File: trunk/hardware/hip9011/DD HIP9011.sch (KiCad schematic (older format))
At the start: 34 parts, among them P1 KNOCK 1, P2 KNOCK 2, P3 12V, P4 CONN_4X2, U1 7805-SOT89, X1 QUARTZ

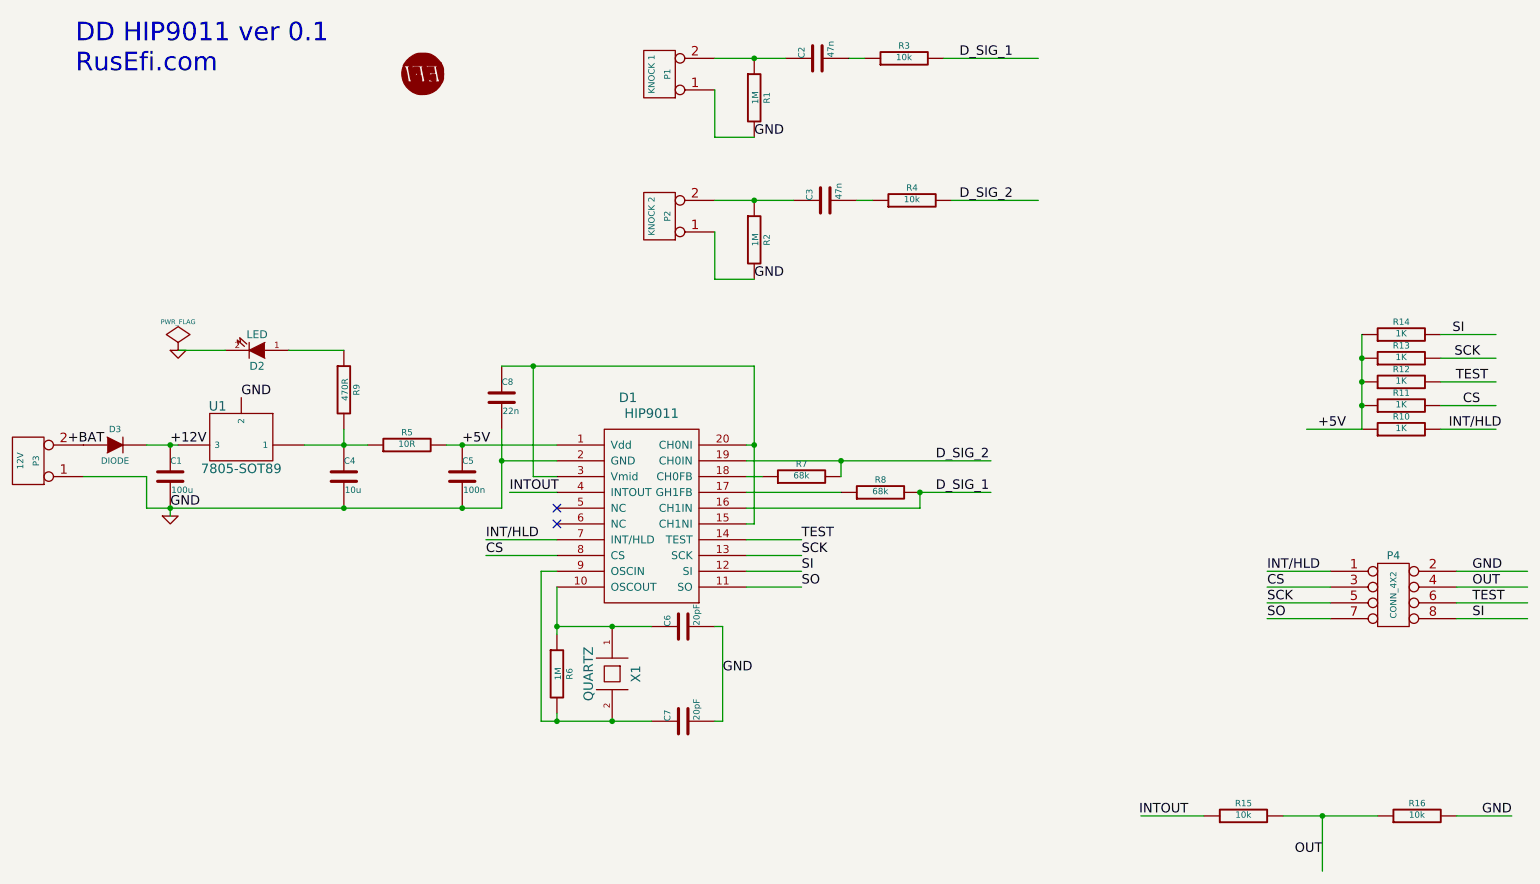
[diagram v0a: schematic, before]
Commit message: proper chip module
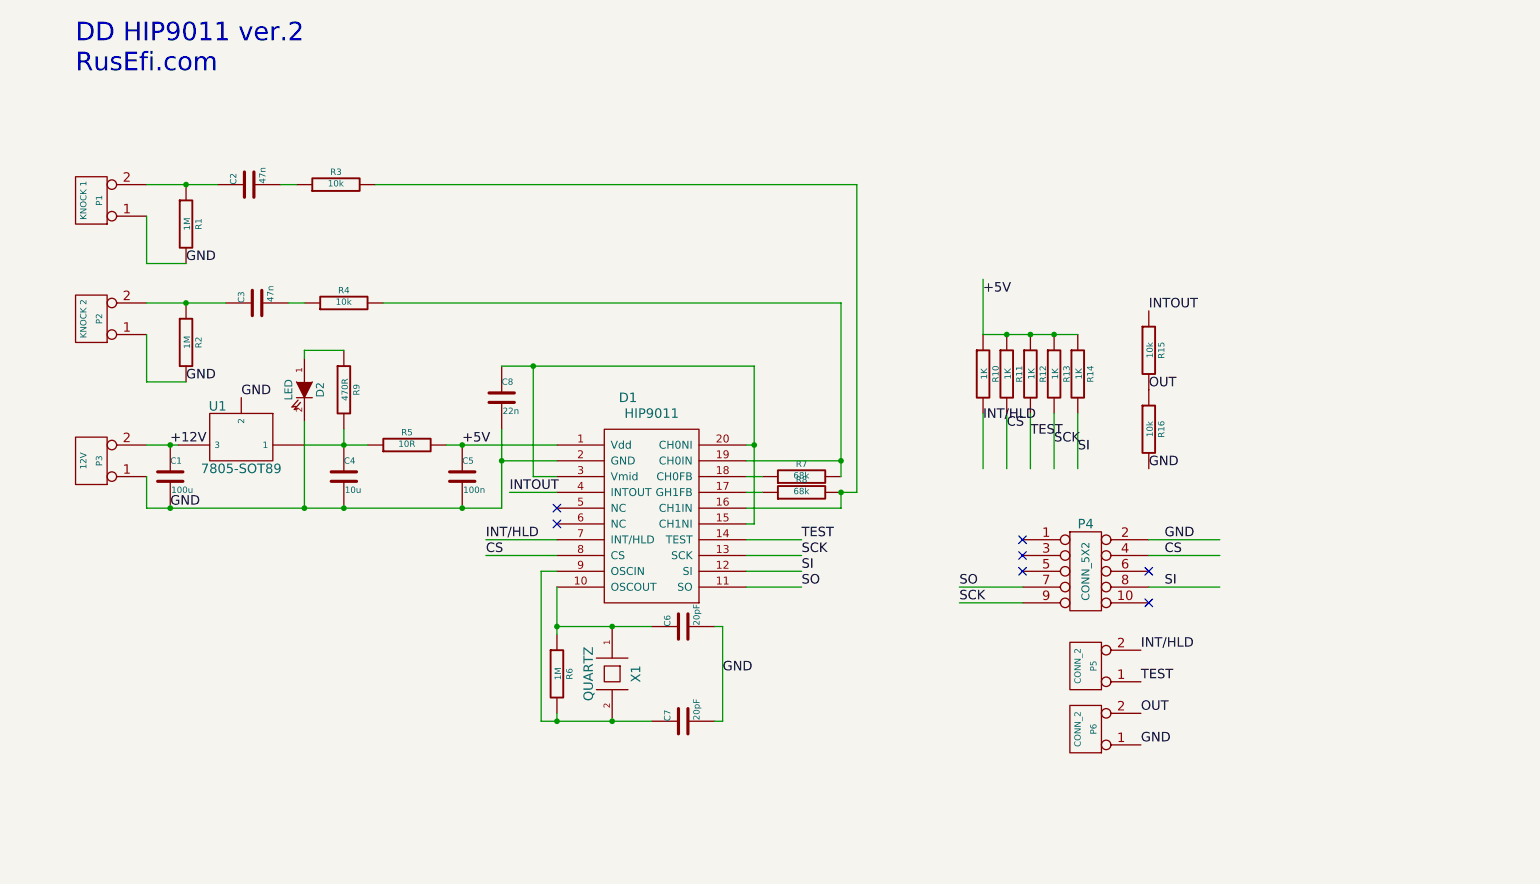
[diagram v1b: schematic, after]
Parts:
- removed D3: DIODE, ~, symbol DIODE
- removed G1: LOGO, symbol LOGO
- removed P4: CONN_4X2, symbol CONN_4X2
- added P4: CONN_5X2, symbol CONN_5X2
- added P5, P6: CONN_2, symbol CONN_2
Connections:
- net labels removed: +BAT, D_SIG_1, D_SIG_2
- wire segments 70 -> 63
- no-connect marks 2 -> 7
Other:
- note added: "DD HIP9011 ver.2\nRusEfi.com"
- note removed: "DD HIP9011 ver 0.1\nRusEfi.com"
- moved on the sheet: C2, C3, D2, P1, P2, P3, R1, R10, R11, R12, R13, R14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
